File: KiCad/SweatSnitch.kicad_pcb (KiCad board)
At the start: 2 copper layers, 37.1 x 59.1 mm, 6 parts, among them U1 HDC1080DMBR, U2 XIAO-RP2040-DIP

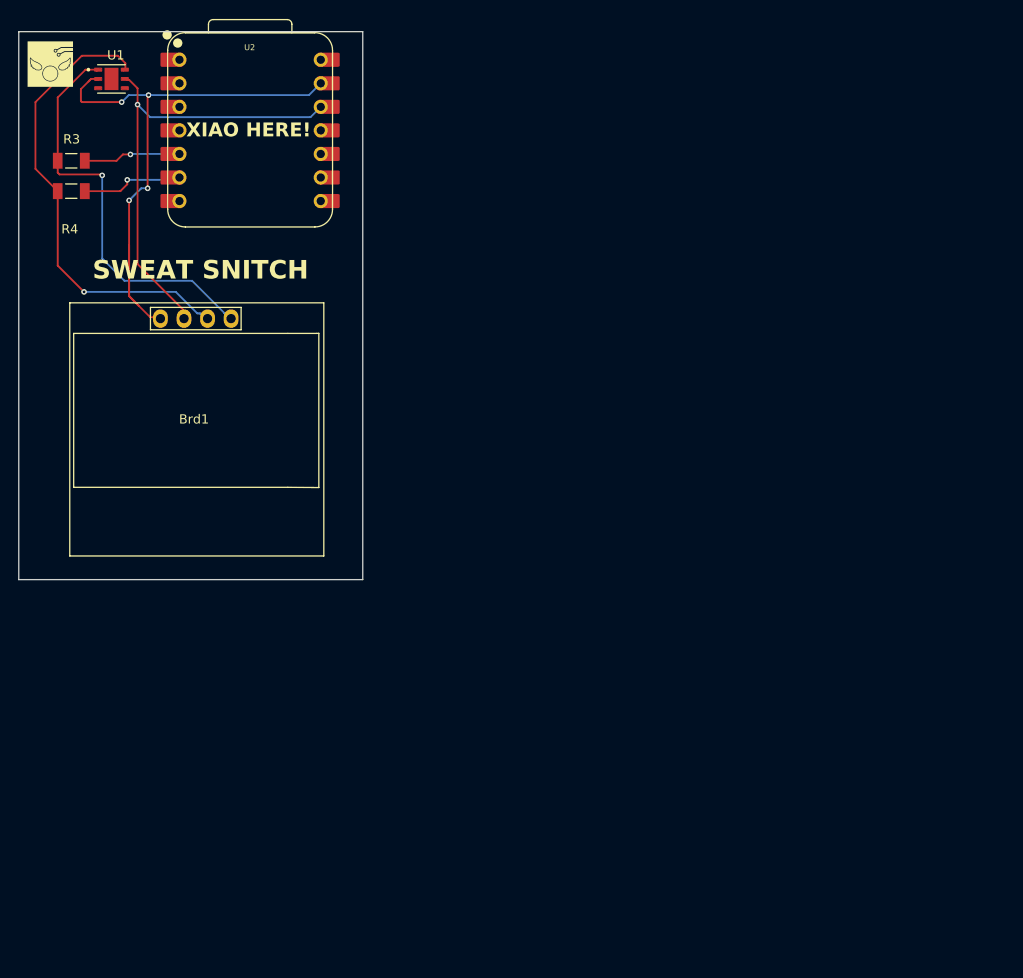
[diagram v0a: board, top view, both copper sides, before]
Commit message: Add files via upload
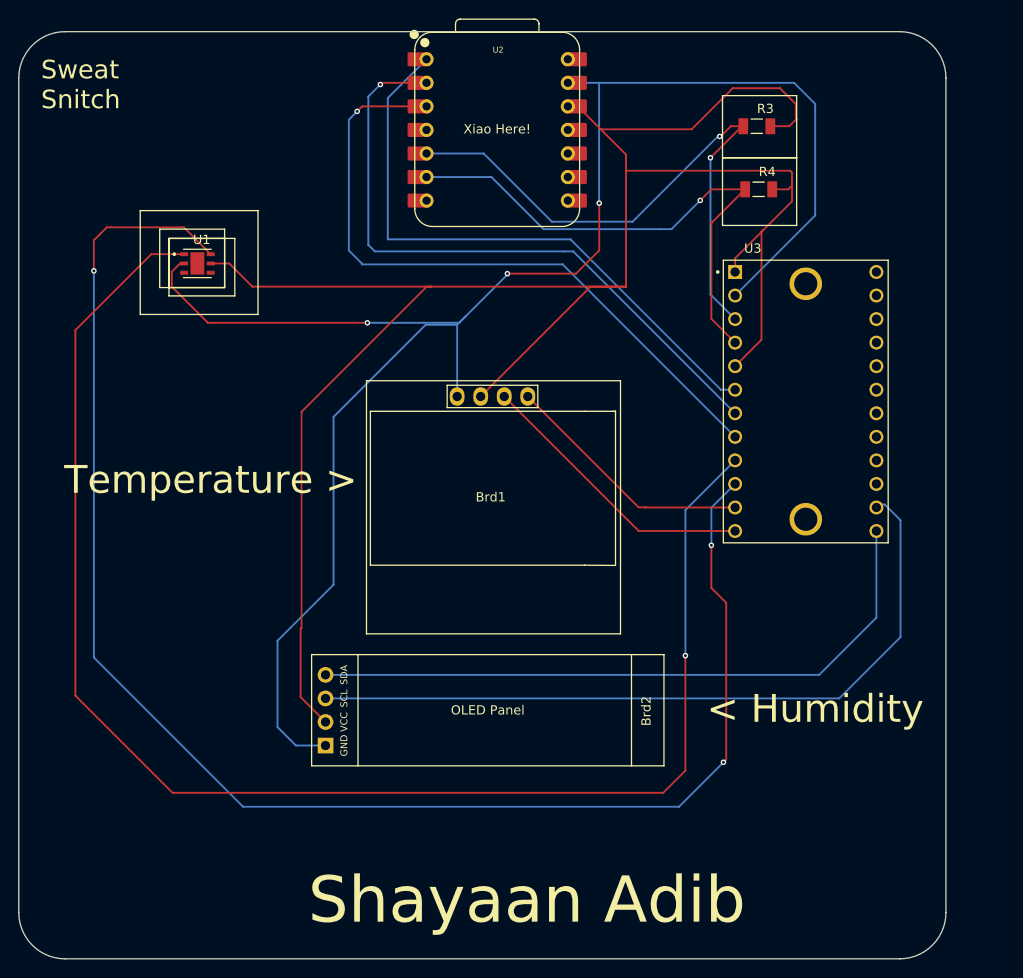
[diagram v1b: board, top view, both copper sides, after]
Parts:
- added Brd2: SSD1306, oled:SSD1306-0.91-OLED-4pin-128x32, F.Cu at (138.3, 170.7)
- added U3: 2717, hii:MODULE_2717, F.Cu at (153.6, 131.4)
- G***: moved to B.Cu
- moved R4 74.1 mm to (148.5, 108.5)
- moved R3 74.0 mm to (148.3, 101.7)
- moved G*** 65.8 mm to (118.7, 141.5), turned to 180 degrees
- moved Brd1 33.1 mm to (119.6, 141.4)
- moved U2 26.6 mm to (120.3, 102.1)
- moved U1 22.0 mm to (88.0, 116.5)
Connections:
- Brd1 pad 3: SCL -> SCL1
- Brd1 pad 4: SDA -> SDA1
- R3 pad 2: Net-(U2-GPIO6/SDA) -> VDD
- R4 pad 2: Net-(U2-GPIO7/SCL) -> VDD
- U1 pad 1: SDA -> SDA0
- U1 pad 6: SCL -> SCL0
- U2 pad 1: unconnected-(U2-GPIO26/ADC0/A0-Pad1) -> A0
- U2 pad 2: unconnected-(U2-GPIO27/ADC1/A1-Pad2) -> A1
- U2 pad 3: unconnected-(U2-GPIO28/ADC2/A2-Pad3) -> A2
- U2 pad 5: Net-(U2-GPIO6/SDA) -> SDA
- U2 pad 6: Net-(U2-GPIO7/SCL) -> SCL
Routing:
- net VDD: track 51.0 -> 222.0 mm, vias 1 -> 0
- net SCL0: track 0.00 -> 167.8 mm, vias 0 -> 3
- net SDA0: track 0.00 -> 161.3 mm, vias 0 -> 1
- net GND: track 66.9 -> 192.8 mm, vias 4 -> 3
- net SCL2: track 0.00 -> 80.8 mm
- net A2: track 0.00 -> 73.1 mm, vias 0 -> 1
- net SDA2: track 0.00 -> 71.3 mm
- net A1: track 0.00 -> 70.0 mm, vias 0 -> 1
- net A0: track 0.00 -> 65.3 mm
- net SCL1: track 0.00 -> 30.9 mm
- net SDA1: track 0.00 -> 27.3 mm
- net SDA: track 45.5 -> 64.9 mm, vias 1 -> 2
- net Net-(U2-GPIO7/SCL): track 11.9 -> 0.00 mm, vias 1 -> 0
- net Net-(U2-GPIO6/SDA): track 11.4 -> 0.00 mm, vias 1 -> 0
- net SCL: track 51.0 -> 57.6 mm
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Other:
- board size 37.1 x 59.1 mm -> 100 x 100 mm
- board text added: "< Humidity"
- board text added: "Shayaan Adib"
- board text added: "Sweat Snitch"
- board text added: "Temperature >"
- board text added: "Xiao Here!"
- board text removed: "SWEAT SNITCH"
- board text removed: "XIAO HERE!"

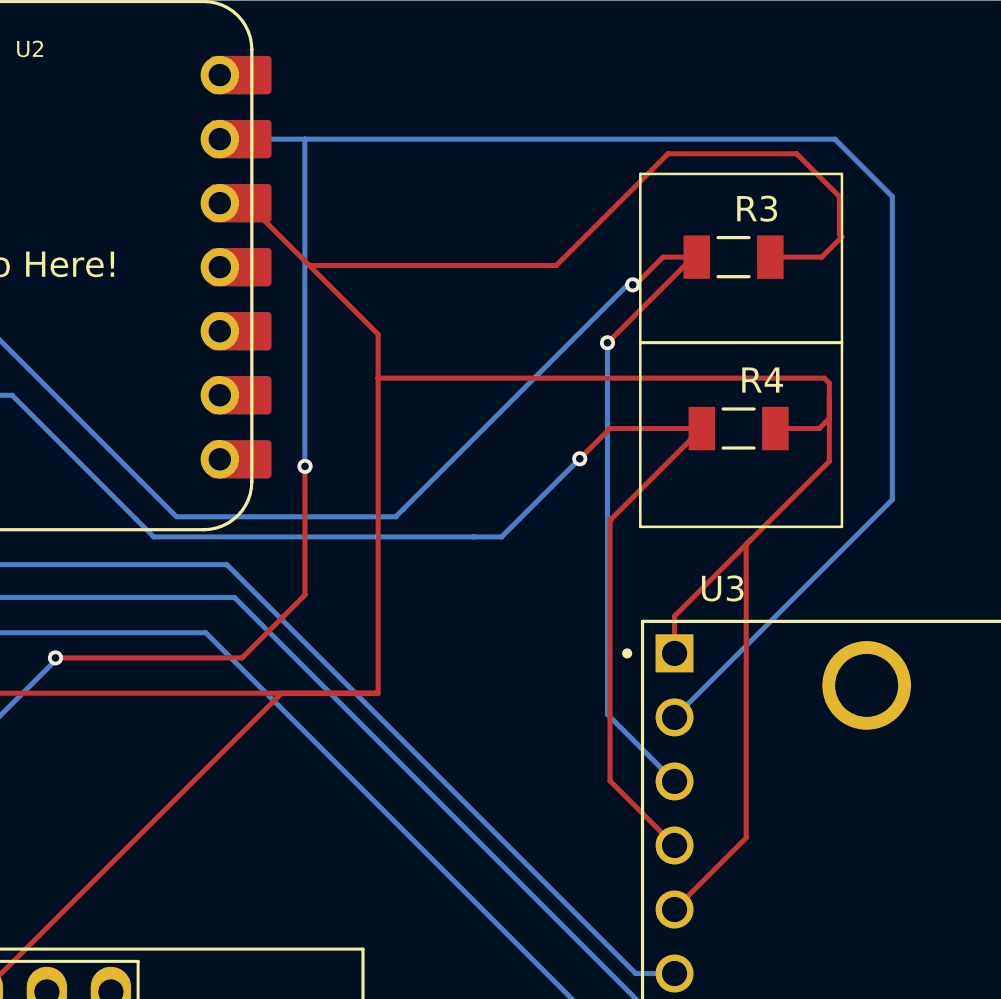
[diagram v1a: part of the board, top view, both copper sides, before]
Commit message: Add files via upload
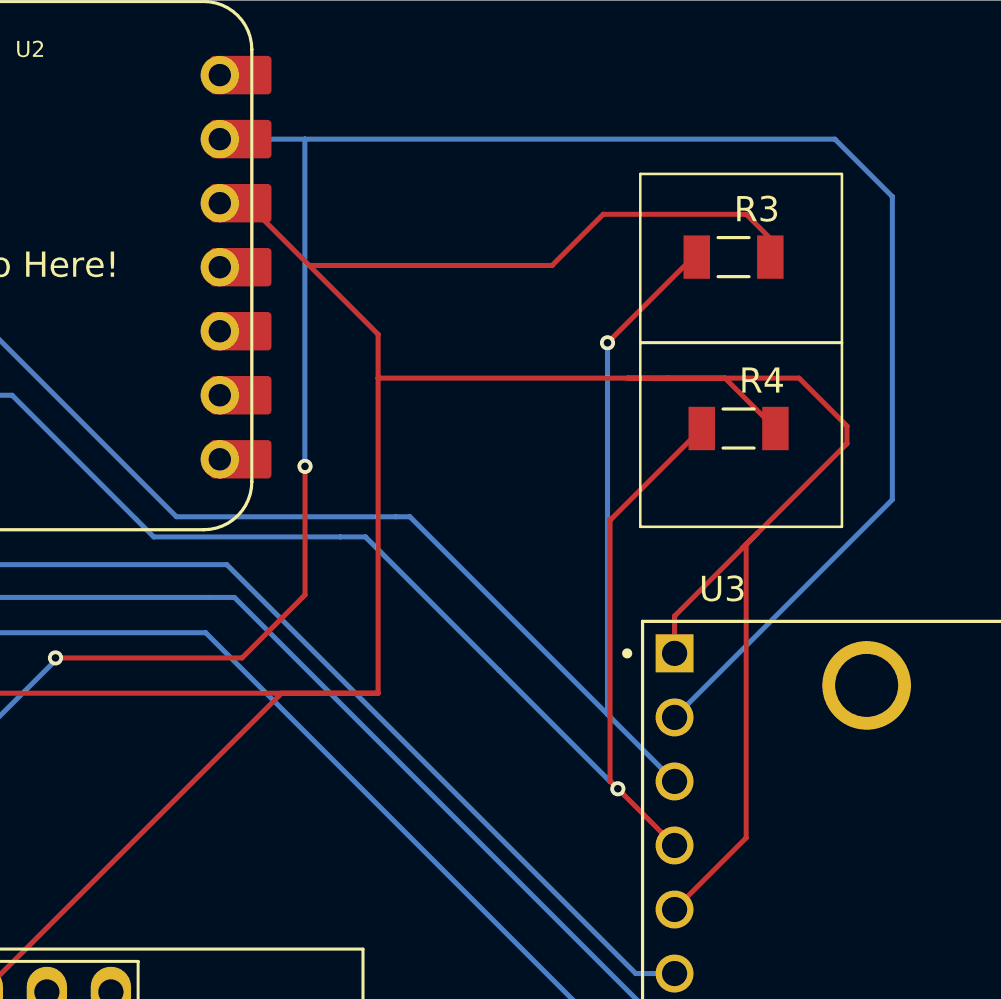
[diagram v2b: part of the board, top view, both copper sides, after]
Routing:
- net SDA: track 64.9 -> 60.6 mm, vias 2 -> 1
- net VDD: track 222.0 -> 218.6 mm
- net SCL: track 57.6 -> 56.6 mm
